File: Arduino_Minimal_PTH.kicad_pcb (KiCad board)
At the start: 2 copper layers, 17.8 x 45.7 mm, 13 parts, among them IC1 ATMEGA328P-PU, P1 I/O lo, P2 FTDI Basic, P3 A4 A5, P4 I/O hi, SW1 Reset, X1 CSTLS16M0X53-B0

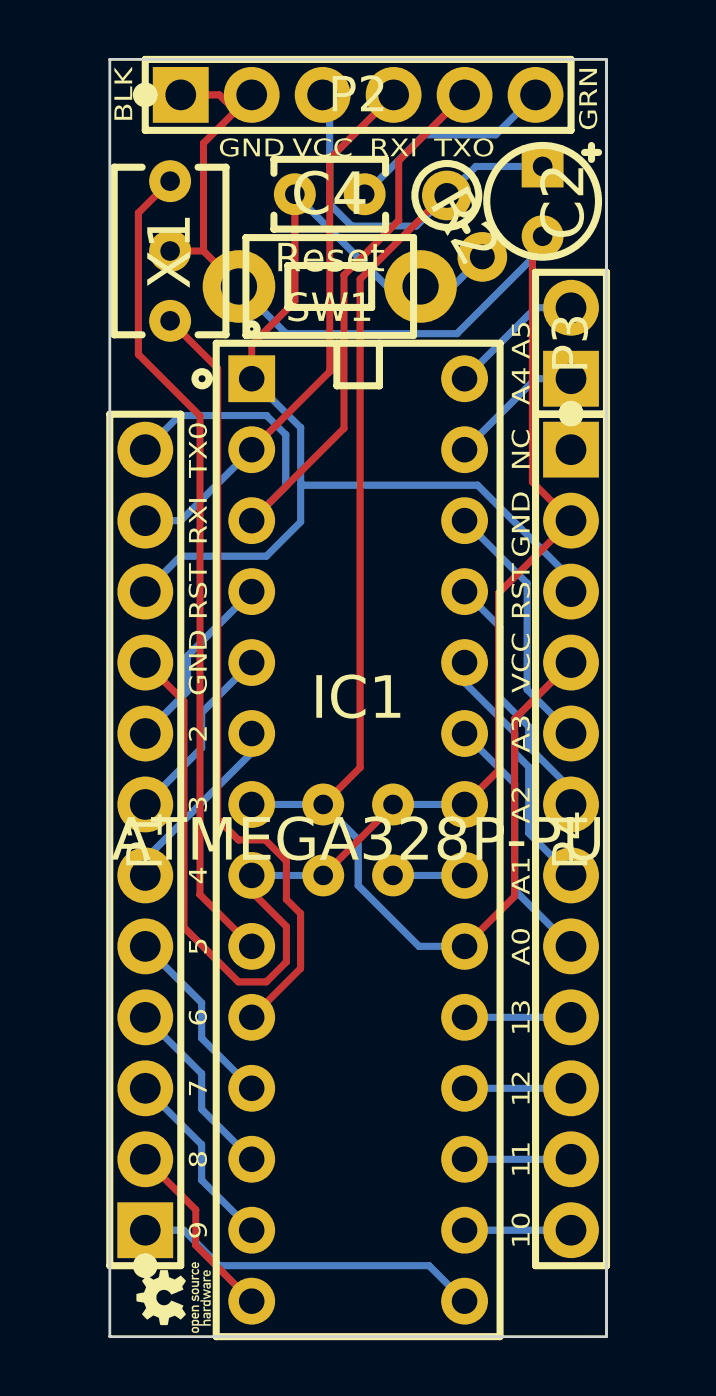
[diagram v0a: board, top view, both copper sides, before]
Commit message: Flooded.
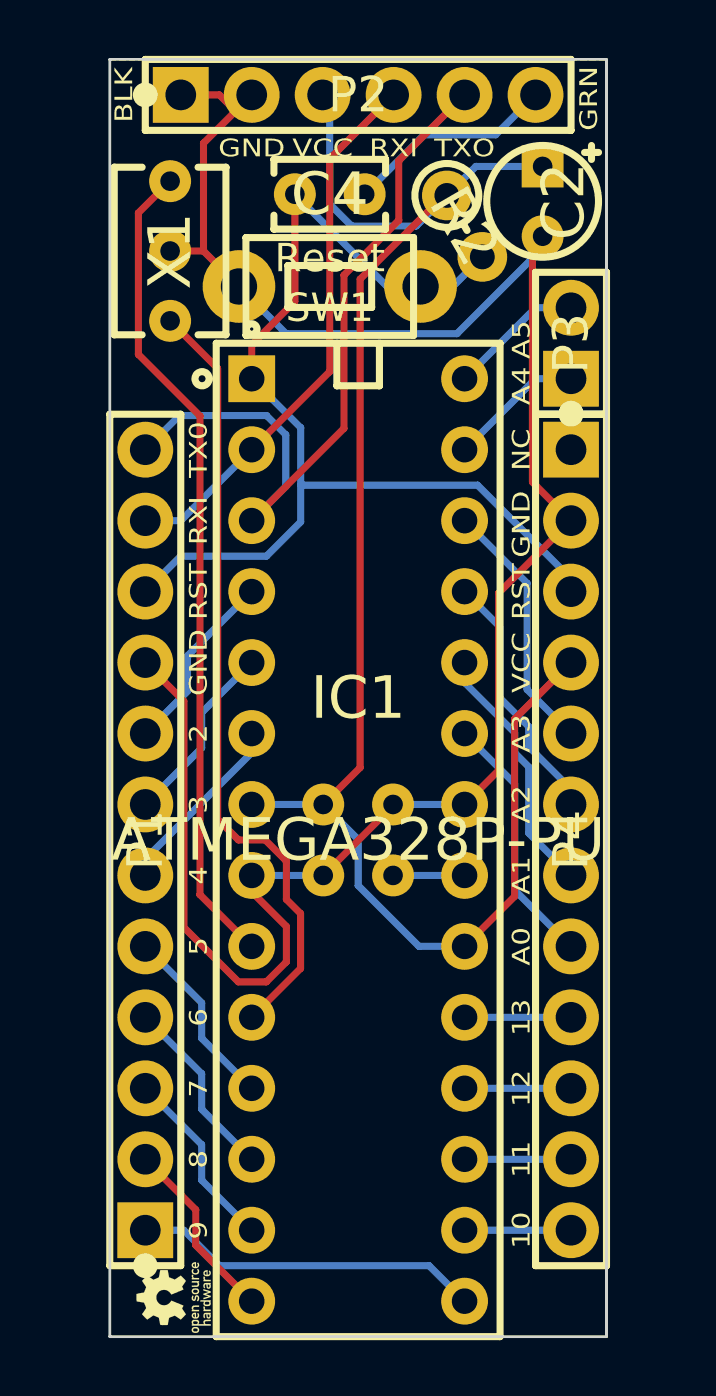
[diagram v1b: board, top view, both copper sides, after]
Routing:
- added copper zone on B.Cu, net GND
- added copper zone on F.Cu, net GND
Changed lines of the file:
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@@
   (segment (start 135.89 109.1997) (end 135.89 110.8501) (width 0.254) (layer B.Cu) (net 27))
   (segment (start 134.6403 107.95) (end 135.89 109.1997) (width 0.254) (layer B.Cu) (net 27))
+  (zone (net 17) (net_name GND) (layer F.Cu) (hatch edge 0.508)
+    (connect_pads (clearance 0.508))
+    (min_thickness 0.2032)
+    (fill (arc_segments 16) (thermal_gap 0.508) (thermal_bridge_width 0.254))
+    (polygon
+      (pts
+        (xy 144.78 127) (xy 127 127) (xy 127 81.28) (xy 144.78 81.28)
+      )
+    )
+  )
+  (zone (net 17) (net_name GND) (layer B.Cu) (hatch edge 0.508)
+    (connect_pads (clearance 0.508))
+    (min_thickness 0.2032)
+    (fill (arc_segments 16) (thermal_gap 0.508) (thermal_bridge_width 0.254))
+    (polygon
+      (pts
+        (xy 144.78 127) (xy 127 127) (xy 127 81.28) (xy 144.78 81.28)
+      )
+    )
+  )
 )

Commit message: Silkscreen optimizations.
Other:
- board text added: "Arduino-compatible Minimal PTH"
- board text removed: "Minimal PTH Arduino-compatible"
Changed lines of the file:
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@@
     (links 47)
     (no_connects 0)
-    (area 124.553134 75.1078 156.260715 137.895001)
+    (area 122.54049 75.1078 156.260715 132.24)
     (thickness 1.6)
     (drawings 40)
@@
     (descr "Non-polar capacitor, 4.0x2.5mm, 2.5mm space, 0.5mm lead")
     (tags "capacitor non-polar bipolar")
-    (fp_text reference C7 (at 0 0 180) (layer B.SilkS)
+    (fp_text reference C7 (at 0 -2.413 180) (layer B.SilkS)
       (effects (font (size 1.524 1.524) (thickness 0.1524)) (justify mirror))
     )
@@
     (descr "Non-polar capacitor, 4.0x2.5mm, 2.5mm space, 0.5mm lead")
     (tags "capacitor non-polar bipolar")
-    (fp_text reference C8 (at 0 0) (layer B.SilkS)
+    (fp_text reference C8 (at 0 -2.159) (layer B.SilkS)
       (effects (font (size 1.524 1.524) (thickness 0.1524)) (justify mirror))
     )
@@
       (xy 0.98552 -0.31496)) (layer F.SilkS) (width 0.00254))
   )
-  (gr_text "Minimal PTH\nArduino-compatible" (at 135.128 112.649 90) (layer B.SilkS)
-    (effects (font (size 1.016 0.889) (thickness 0.2032)) (justify left mirror))
-  )
-  (gr_circle (center 130.302 92.71) (end 130.302 92.456) (layer F.SilkS) (width 0.254))
+  (gr_circle (center 130.302 92.71) (end 130.556 92.71) (layer F.SilkS) (width 0.254))
+  (gr_text "Arduino-compatible\nMinimal PTH\n" (at 135.255 91.44 90) (layer B.SilkS)
+    (effects (font (size 1.27 0.8382) (thickness 0.2032)) (justify left mirror))
+  )
   (gr_text A5 (at 141.732 91.313 90) (layer F.SilkS)
     (effects (font (size 0.635 0.762) (thickness 0.1524)))
